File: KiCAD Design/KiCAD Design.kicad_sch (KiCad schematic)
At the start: 60 parts, among them J1 USB_B_Micro, J2 Conn_01x04_Pin, J5 Micro_SD_Card, SW1 SW_SPDT, U1 STM32F103C8Tx, U2 AMS1117-3.3, U3 BNO055, U4 L80-R, U5 nRF24L01P, Y1 16MHz, Y2 16MHz

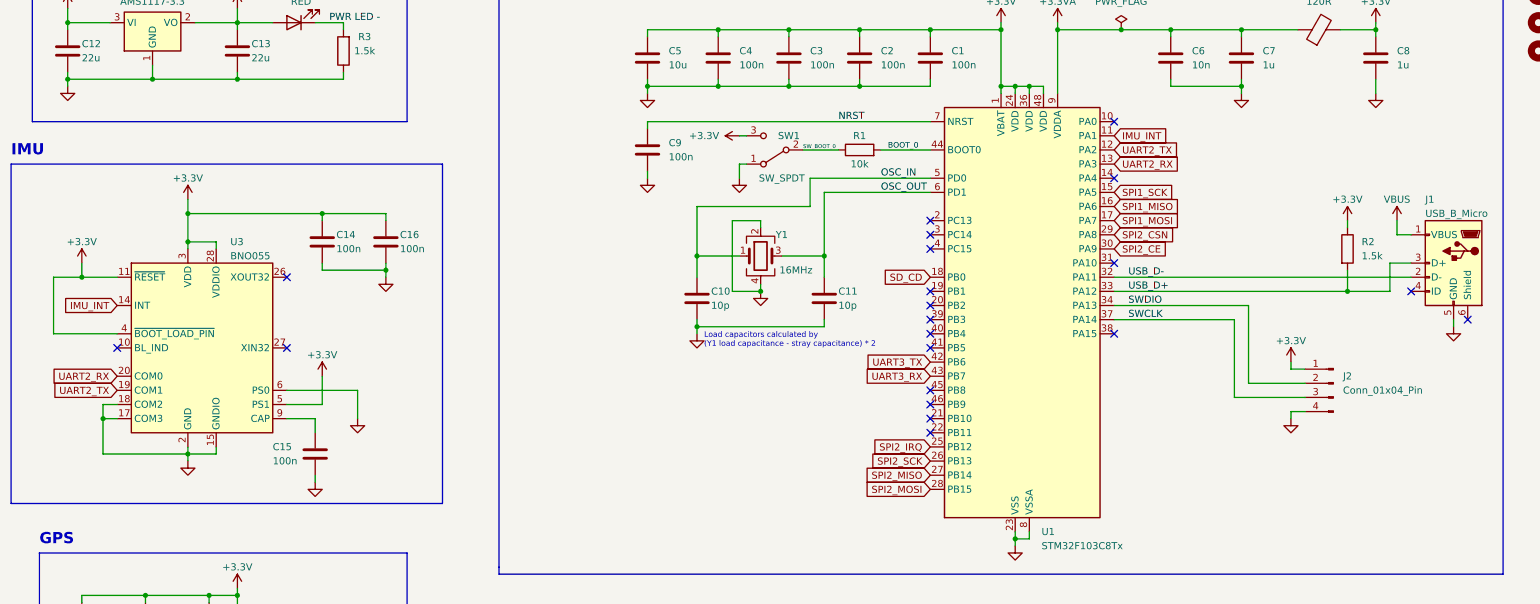
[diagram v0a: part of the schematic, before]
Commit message: Assembly files
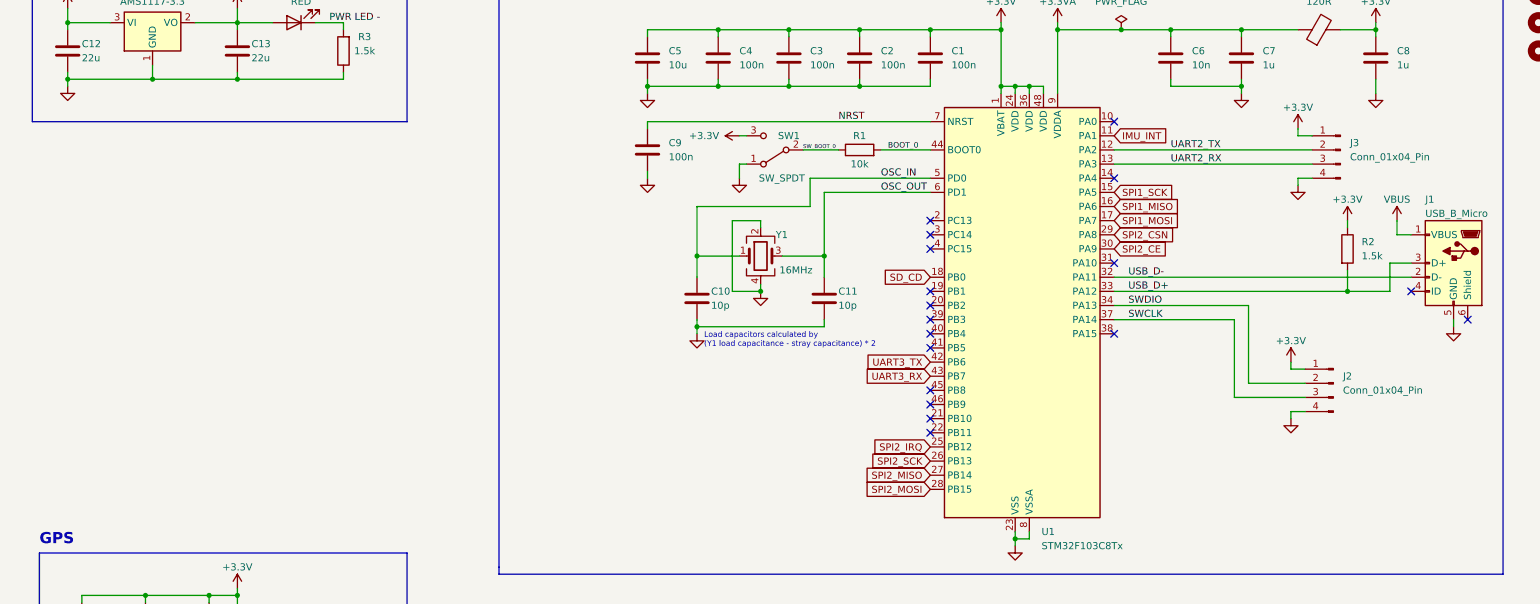
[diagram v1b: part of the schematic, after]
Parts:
- removed C14, C15, C16: 100n, Capacitor_SMD:C_0402_1005Metric, symbol Device:C
- removed U3: BNO055, Package_LGA:LGA-28_5.2x3.8mm_P0.5mm, symbol Sensor_Motion:BNO055
- added J3: Conn_01x04_Pin, Connector_PinHeader_2.54mm:PinHeader_1x04_P2.54mm_Vertical, symbol Connector:Conn_01x04_Pin
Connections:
- net +3.3V: now also J3.1 (Pin_1)
- net GND: now also J3.4 (Pin_4)
- net UART2_RX: now also J3.3 (Pin_3)
- net UART2_TX: now also J3.2 (Pin_2)
- no-connect marks 28 -> 25
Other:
- note removed: "IMU"
